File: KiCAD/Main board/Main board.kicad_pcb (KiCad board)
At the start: 2 copper layers, 150 x 170 mm, 239 parts, among them J1 Conn_01x03, J10 GPIO 0, J11 GPIO 1, J12 Conn_01x03, J13 Conn_01x02, J14 Conn_01x02, J2 Conn_01x03, J3 Conn_01x02, J4 Conn_01x03, J5 Conn_01x02, J6 Conn_01x03, J7 Conn_01x03, J8 Conn_01x03, J9 Conn_01x03, U1 PCM1789, U11 PCM1789, U18 12V, U19 5V, U2 LM4562, U20 8V, U21 15V, U23 LIN_REG_±5V, U24 LIN_REG_±12V, U25 LIN_REG_±5V, U26 LIN_REG_±12V, U27 PCM1804, U28 PCM1804, U7 PCM1789, U9 LM4562

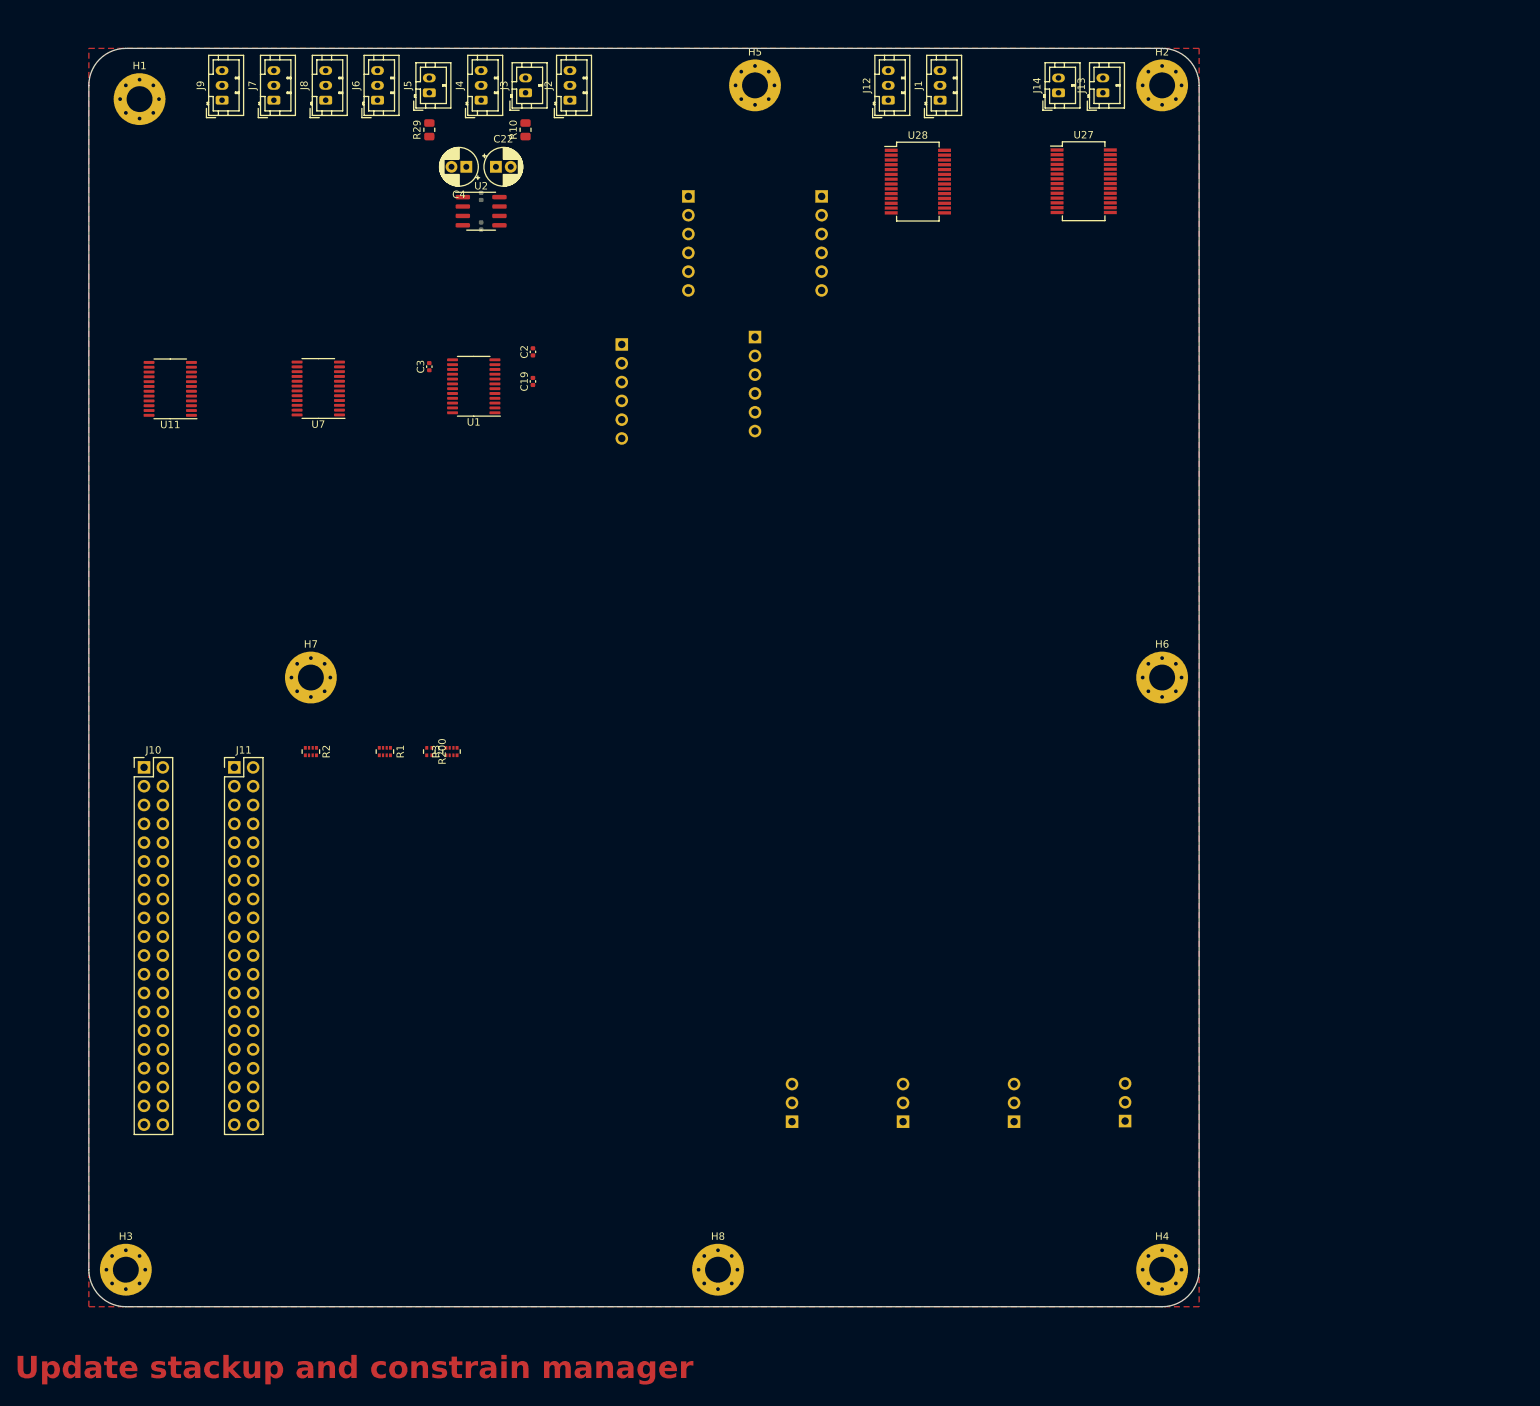
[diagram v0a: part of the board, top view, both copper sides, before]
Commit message: Updated main board
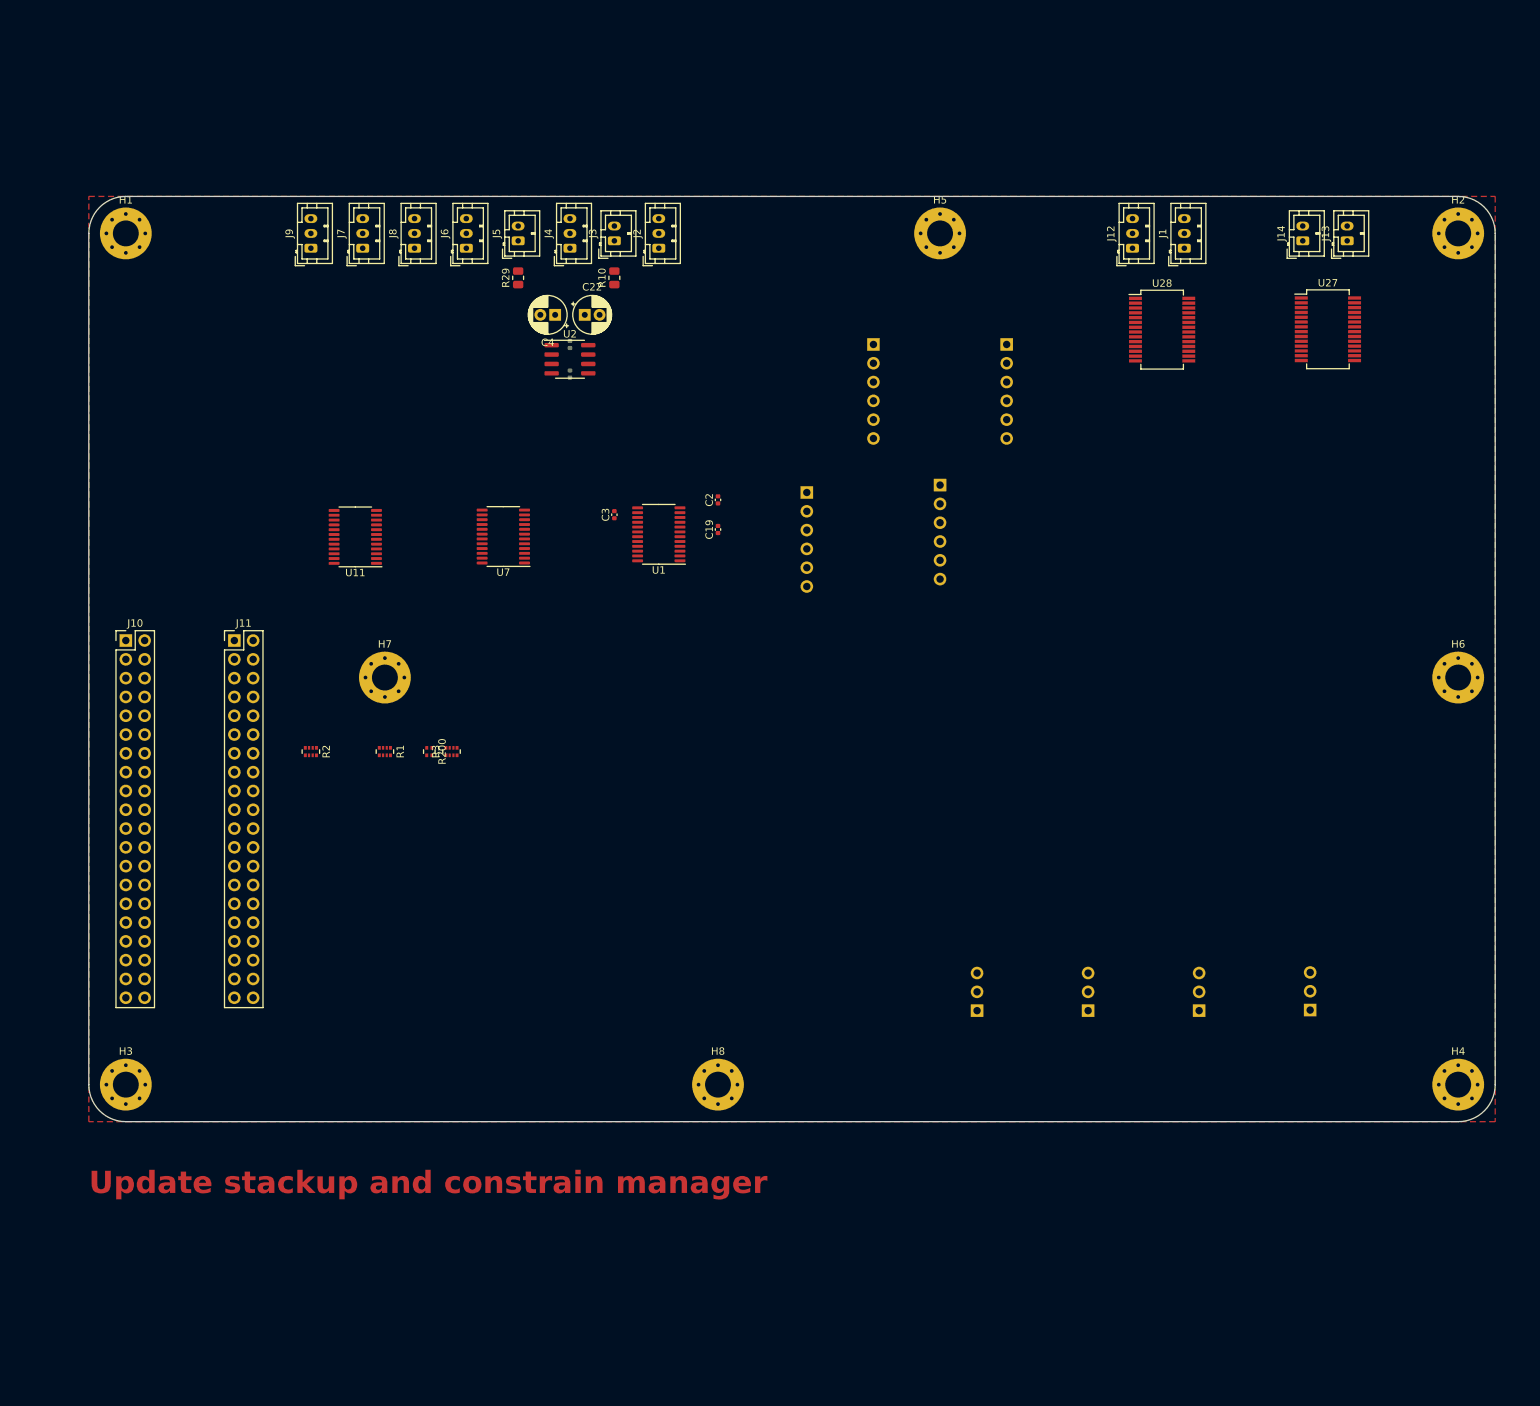
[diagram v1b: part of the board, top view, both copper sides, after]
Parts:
- moved H4 47.2 mm to (235.0, 220.0)
- moved H2 44.7 mm to (235.0, 105.0)
- moved H6 40.0 mm to (235.0, 165.0)
- moved J1 38.6 mm to (198.0, 107.0)
- moved J12 38.6 mm to (191.0, 107.0)
- moved J13 38.6 mm to (220.0, 106.0)
- moved J14 38.6 mm to (214.0, 106.0)
- moved U27 38.6 mm to (217.4, 118.0)
- moved U28 38.6 mm to (195.0, 118.0)
- moved C19 32.0 mm to (135.0, 145.0)
- moved C2 32.0 mm to (135.0, 141.0)
- moved C3 32.0 mm to (121.0, 143.0)
- moved H5 32.0 mm to (165.0, 105.0)
- moved U1 32.0 mm to (127.0, 145.7)
- moved U11 32.0 mm to (86.0, 146.0)
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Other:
- board size 150 x 170 mm -> 190 x 125 mm
